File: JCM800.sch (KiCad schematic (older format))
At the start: 114 parts, among them U1 ECC83, U2 ECC83, U3 ECC83, U4 EL84, U5 EL84

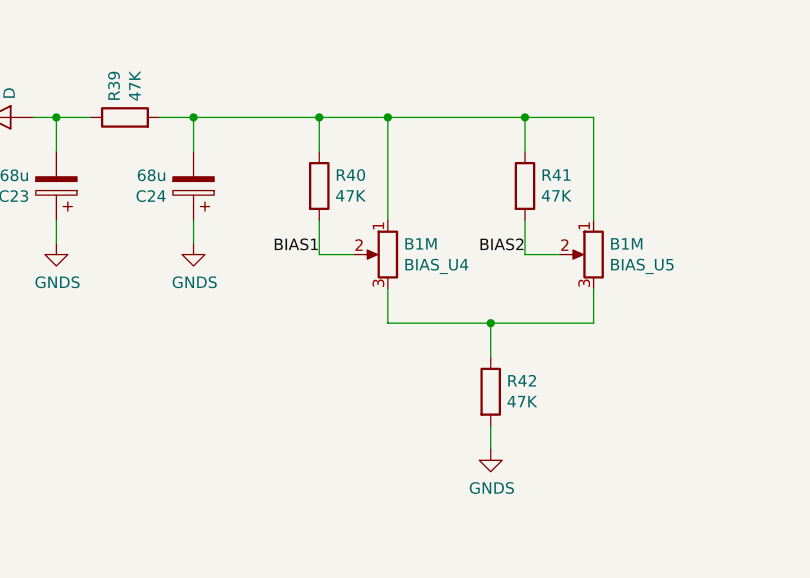
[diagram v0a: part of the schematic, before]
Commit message: Tweaks
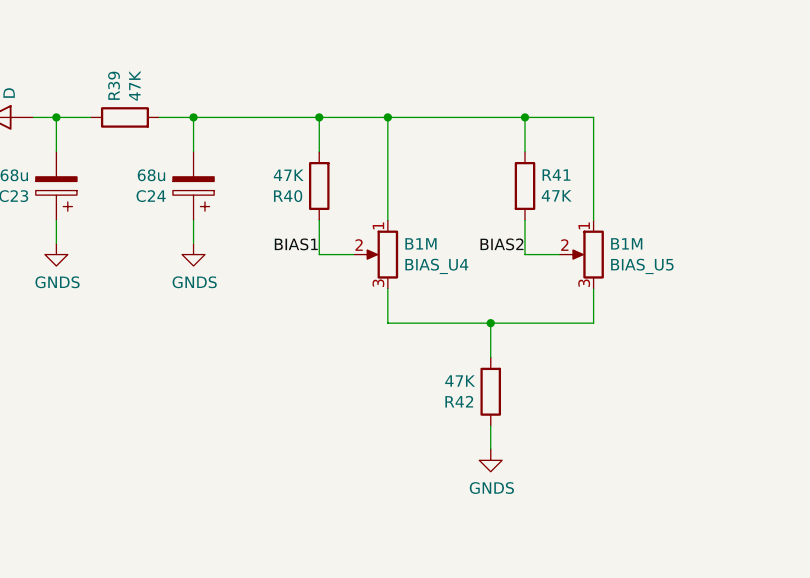
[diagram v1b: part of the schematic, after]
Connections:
- net BIAS1: now also R40.1; no longer R40.2
- net GNDS: now also R42.1; no longer R42.2
- net at BIAS_U4.1, BIAS_U5.1, C24.2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: now also R40.2; no longer R40.1
- net at BIAS_U4.3, BIAS_U5.3: now also R42.2; no longer R42.1
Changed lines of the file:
@@
 F 3 "~" H 13750 8900 50  0001 C CNN
 	1    13750 8900
-	1    0    0    -1
+	-1   0    0    1
 $EndComp
 Wire Wire Line
@@
 Wire Wire Line
 	12450 7700 13000 7700
-$Comp
-L Device:R R41
-U 1 1 5E0B73F7
-P 13900 8000
-F 0 "R41" H 13970 8046 50  0000 L CNN
-F 1 "47K" H 13970 7955 50  0000 L CNN
-F 2 "Resistor_THT:R_Axial_DIN0207_L6.3mm_D2.5mm_P10.16mm_Horizontal" V 13830 8000 50  0001 C CNN
-F 3 "~" H 13900 8000 50  0001 C CNN
-	1    13900 8000
-	1    0    0    -1
-$EndComp
-$Comp
-L Device:R R40
-U 1 1 5E0B6F27
-P 13000 8000
-F 0 "R40" H 13070 8046 50  0000 L CNN
-F 1 "47K" H 13070 7955 50  0000 L CNN
-F 2 "Resistor_THT:R_Axial_DIN0207_L6.3mm_D2.5mm_P10.16mm_Horizontal" V 12930 8000 50  0001 C CNN
-F 3 "~" H 13000 8000 50  0001 C CNN
-	1    13000 8000
-	1    0    0    -1
-$EndComp
 Text Label 7400 8150 0    50   ~ 0
 BIAS1
@@
 	1    0    0    1
 $EndComp
+$Comp
+L Device:R R41
+U 1 1 5E0B73F7
+P 13900 8000
+F 0 "R41" H 13970 8046 50  0000 L CNN
+F 1 "47K" H 13970 7955 50  0000 L CNN
+F 2 "Resistor_THT:R_Axial_DIN0207_L6.3mm_D2.5mm_P10.16mm_Horizontal" V 13830 8000 50  0001 C CNN
+F 3 "~" H 13900 8000 50  0001 C CNN
+	1    13900 8000
+	1    0    0    -1
+$EndComp
+$Comp
+L Device:R R40
+U 1 1 5E0B6F27
+P 13000 8000
+F 0 "R40" H 13070 8046 50  0000 L CNN
+F 1 "47K" H 13070 7955 50  0000 L CNN
+F 2 "Resistor_THT:R_Axial_DIN0207_L6.3mm_D2.5mm_P10.16mm_Horizontal" V 12930 8000 50  0001 C CNN
+F 3 "~" H 13000 8000 50  0001 C CNN
+	1    13000 8000
+	-1   0    0    1
+$EndComp
 $EndSCHEMATC
